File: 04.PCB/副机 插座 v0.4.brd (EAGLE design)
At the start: 36.8 x 45.4 mm, 26 parts, among them Y2 RESONATORSMD

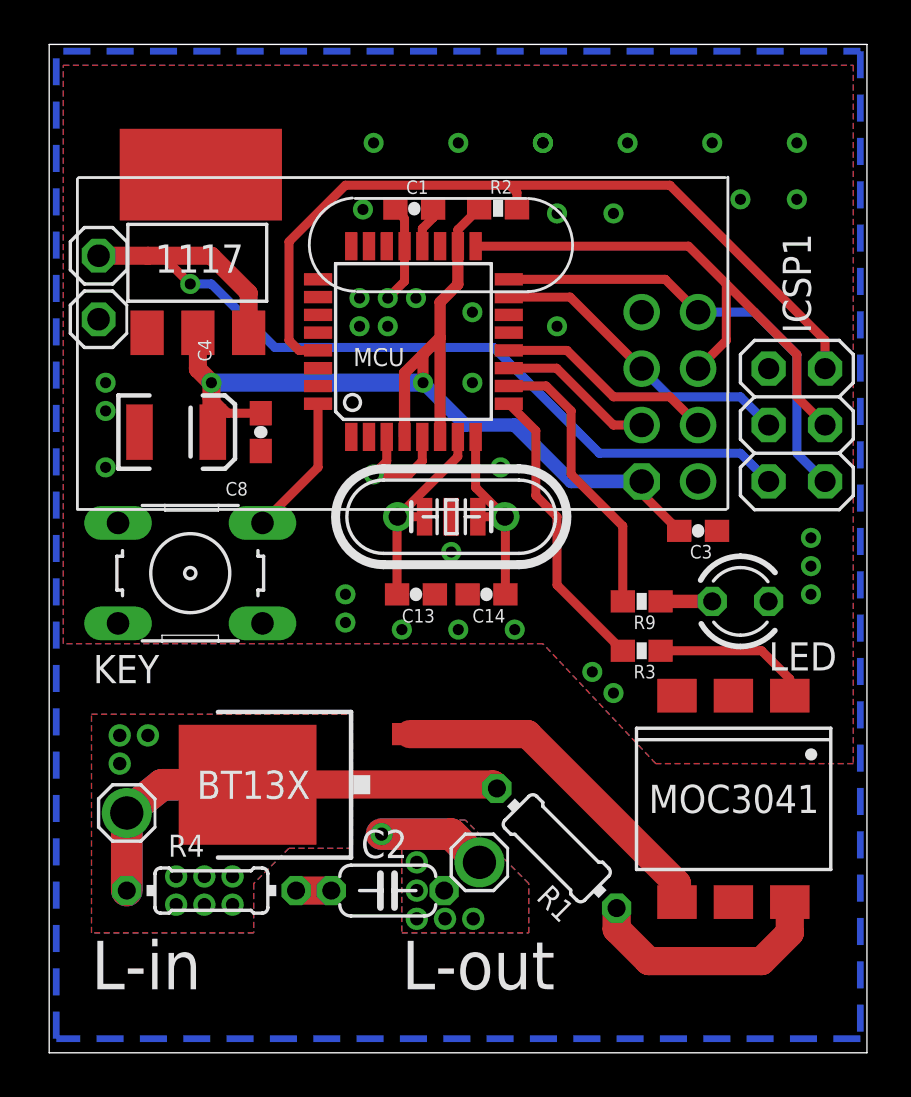
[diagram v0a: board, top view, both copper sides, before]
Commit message: 更新了几个新pcb
更新了几个新pcb
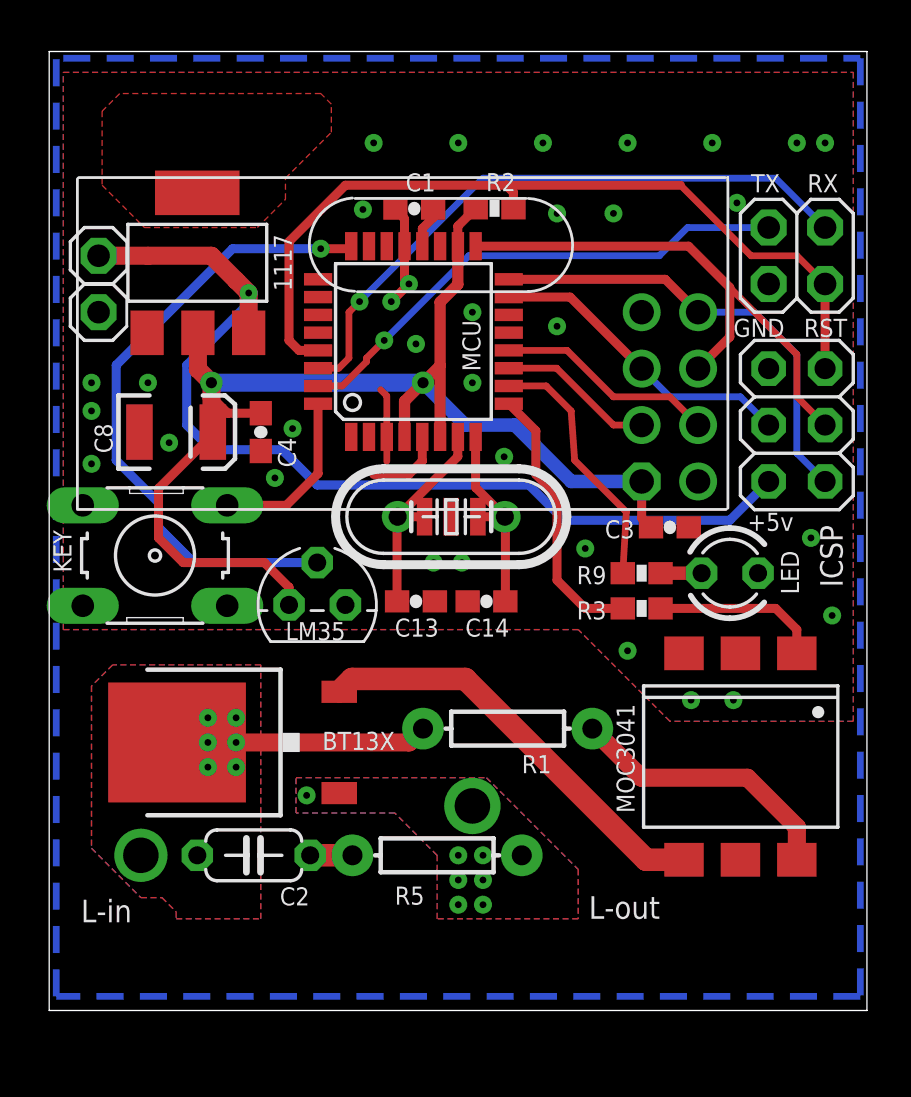
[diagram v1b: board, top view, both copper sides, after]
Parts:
- removed R4: 100, resistor:0204/7
- removed U$1, U$2: (no value), PKJ:PIN1
- added JP1: (no value), pinhead:2X02
- added LM35: (no value), transistor-neu-to92:TO92-E1
- added R5: 100, MY3:AXIAL-0.3
- 1117: device burr-brown:SOT223 -> MY3:SOT223
- R1: device resistor:0204/7 -> MY3:AXIAL-0.3
- moved C2 6.24 mm to (9.84, 9.84)
- moved R1 5.82 mm to (21.3, 15.5), turned to 180 degrees
- moved BT13X 3.70 mm to (8.89, 14.9)
- moved MOC3041 1.93 mm to (31.8, 14.3)
- moved R3 1.90 mm to (27.3, 21.0)
- moved KEY 1.77 mm to (5.40, 23.3)
- moved LED 1.36 mm to (31.3, 22.5)
- moved C3 1.28 mm to (28.6, 24.6)
- moved R9 1.27 mm to (27.3, 22.5)
- moved U$4 0.32 mm to (2.86, 34.3)
- moved C13 0.32 mm to (17.1, 21.3)
- moved C14 0.32 mm to (20.3, 21.3)
- moved R2 0.16 mm to (20.7, 39.0)
- renumbered ICSP1 to ICSP
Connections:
- removed net N$6: C2.2, R4.2
- new net N$3: C2.1, R5.P$1
- net A1: now also LM35.2
- net D0/RXI: now also JP1.4
- net D1/TXO: now also JP1.2
- net GND: now also JP1.1, LM35.3
- net IN: now also C2.2, R1.P$2; no longer R1.2, R4.1, U$2.1
- net N$1: now also R1.P$1; no longer R1.1
- net OUT: now also R5.P$2; no longer C2.1, U$1.1
- net RESET: now also JP1.3
- net VCC: now also 1117.4, LM35.1
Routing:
- net A1: track 0.00 -> 28.7 mm, vias 0 -> 1
- net D0/RXI: track 0.00 -> 28.5 mm, vias 0 -> 1
- net D1/TXO: track 0.00 -> 23.3 mm, vias 0 -> 1
- net IN: track 30.1 -> 11.3 mm, vias 10 -> 7
- net OUT: track 11.1 -> 0.00 mm, vias 7 -> 8
- net VCC: track 49.3 -> 60.0 mm
- net N$14: track 161.0 -> 156.5 mm
- net VIN: track 41.4 -> 45.7 mm
- net N$2: track 15.6 -> 19.1 mm
- net N$3: track 0.00 -> 1.90 mm
- net N$6: track 1.59 -> 0.00 mm
- net RESET: track 36.5 -> 38.0 mm
- net D2/INT0: track 6.40 -> 7.82 mm
- net GND: track 10.0 -> 11.4 mm, vias 36 -> 33
- net N$1: track 11.2 -> 12.5 mm
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- added copper zone on layer 1, net VCC
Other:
- board size 36.8 x 45.4 mm -> 36.8 x 43.2 mm
- board text added: "+5v"
- board text added: "G"
- board text added: "GND"
- board text added: "RST"
- board text added: "RX"
- board text added: "TX"
- board text removed: "v"
